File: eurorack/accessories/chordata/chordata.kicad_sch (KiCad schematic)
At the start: 44 parts, among them J1 USB_C_Receptacle_USB2.0, J2 Conn_02x05_Odd_Even, J3 Conn_01x18, J4 Conn_01x18, SW1 SW_Push, SW2 SW_Push, U1 MIC5219-3.3YM5, U2 RP2040, U3 W25Q128JVS, Y1 Crystal_GND24

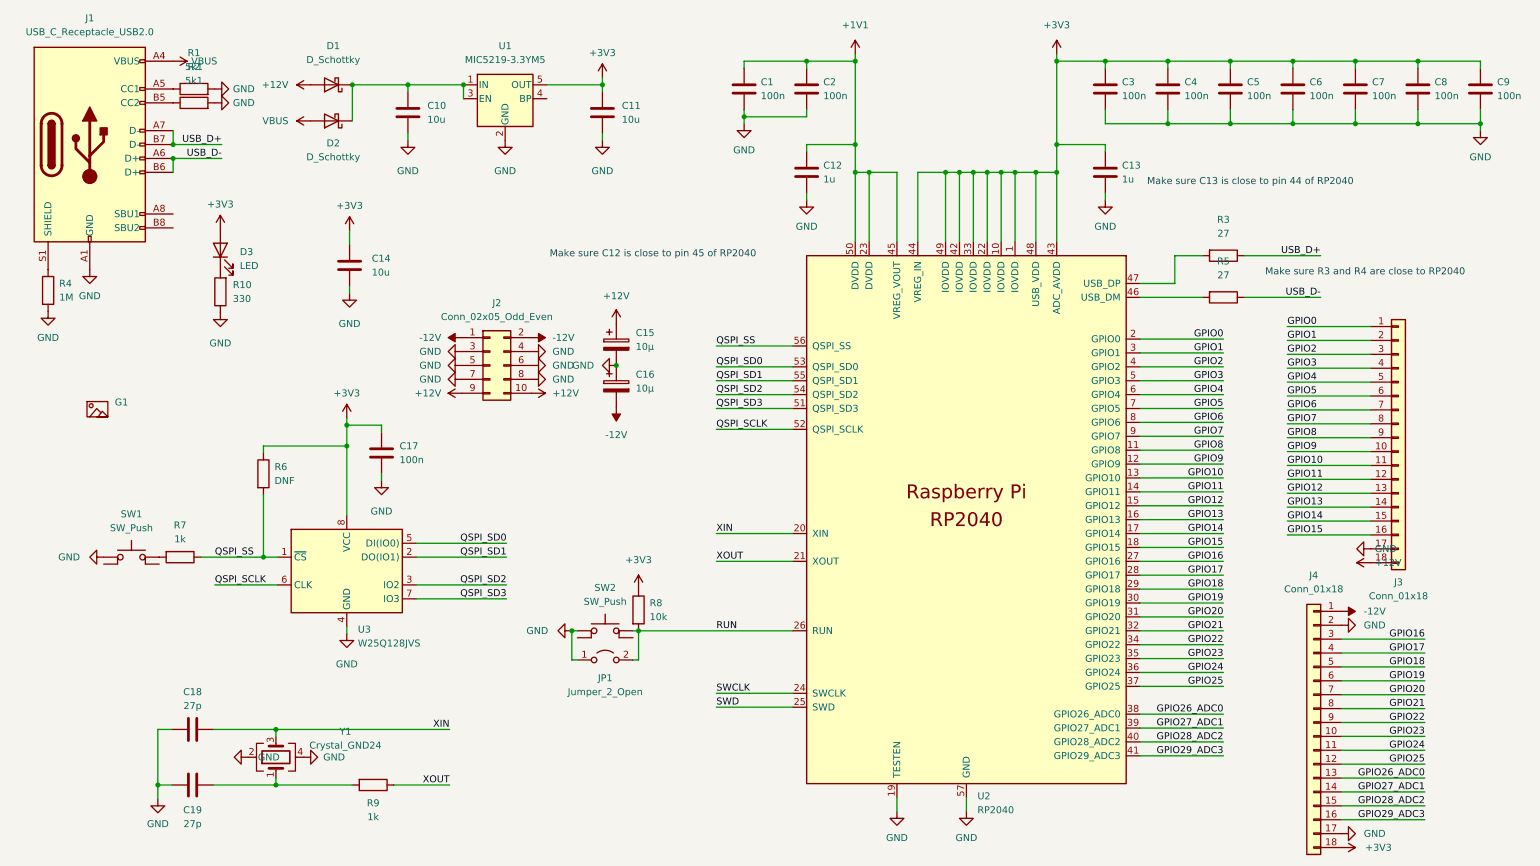
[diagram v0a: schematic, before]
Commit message: final chordata v1 layout
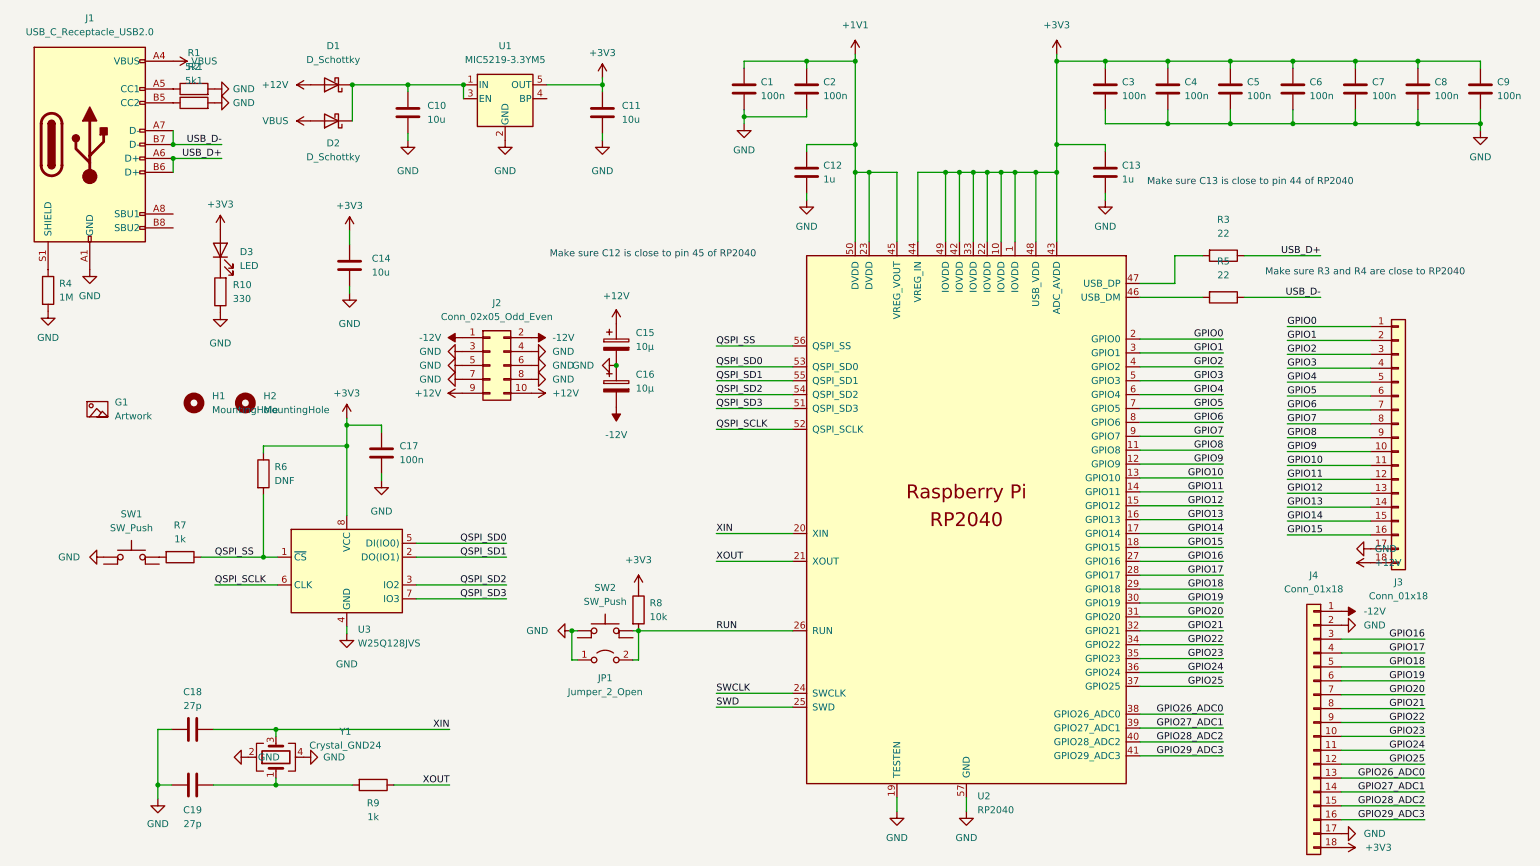
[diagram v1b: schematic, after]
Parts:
- added H1, H2: MountingHole, Pale Slim Ghost:hole JLCPCB tooling, symbol Mechanical:MountingHole
- C15, C16, J1, J2, J3, J4, JP1, R6, U1: now left out of the parts list
- D3: footprint LED_SMD:LED_0402_1005Metric -> LED_SMD:LED_0603_1608Metric
- G1: value (none) -> Artwork; footprint (none) -> Pale Slim Ghost:logo 12mm
- R3, R5: value 27 -> 22
- SW1, SW2: footprint Pale Slim Ghost:SW_Push_1P1T_NO_CK_KMR2 -> Pale Slim Ghost:SW_Push_1P1T_SKSGACE010; now left out of the parts list
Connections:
- net USB_D+: now also J1.A6 (D+), J1.B6 (D+); no longer J1.A7 (D-), J1.B7 (D-)
- net USB_D-: now also J1.A7 (D-), J1.B7 (D-); no longer J1.A6 (D+), J1.B6 (D+)

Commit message: chordata v2 final layout
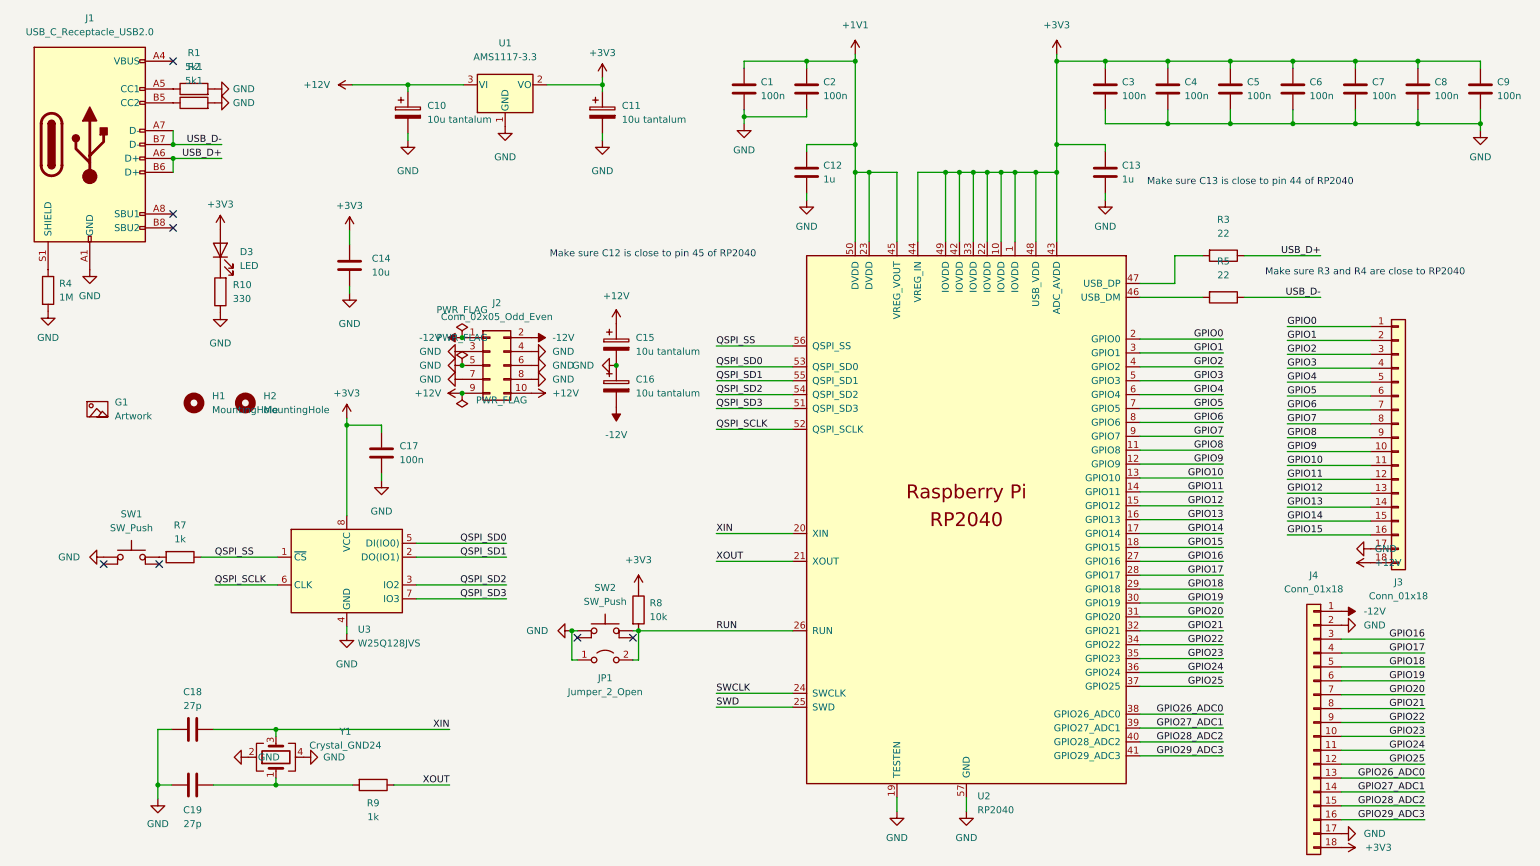
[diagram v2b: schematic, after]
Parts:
- removed C10: 10u, Capacitor_SMD:C_0805_2012Metric, symbol Device:C
- removed D1, D2: D_Schottky, Diode_SMD:D_SOD-123, symbol Device:D_Schottky
- removed R6: DNF, Resistor_SMD:R_0402_1005Metric, symbol Device:R
- removed U1: MIC5219-3.3YM5, Package_TO_SOT_SMD:SOT-23-5, symbol Regulator_Linear:MIC5219-3.3YM5
- added C10: 10u tantalum, Capacitor_Tantalum_SMD:CP_EIA-3216-18_Kemet-A, symbol Device:C_Polarized
- added U1: AMS1117-3.3, Package_TO_SOT_SMD:SOT-223-3_TabPin2, symbol Regulator_Linear:AMS1117-3.3
- C11: value 10u -> 10u tantalum; footprint Capacitor_SMD:C_0805_2012Metric -> Capacitor_Tantalum_SMD:CP_EIA-3216-18_Kemet-A; symbol Device:C -> Device:C_Polarized
- C15, C16: value 10μ -> 10u tantalum; footprint Capacitor_SMD:CP_Elec_5x4.5 -> Capacitor_Tantalum_SMD:CP_EIA-3216-18_Kemet-A; now in the parts list
- J1: footprint Connector_USB:USB_C_Receptacle_XKB_U262-16XN-4BVC11 -> Connector_USB:USB_C_Receptacle_GCT_USB4085
- SW1, SW2: footprint Pale Slim Ghost:SW_Push_1P1T_SKSGACE010 -> Pale Slim Ghost:SW_Push_1P1T_NO_CK_KMR2
- U2: footprint Package_DFN_QFN:QFN-56-1EP_7x7mm_P0.4mm_EP5.6x5.6mm_ThermalVias -> Package_DFN_QFN:QFN-56-1EP_7x7mm_P0.4mm_EP3.2x3.2mm_ThermalVias
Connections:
- net +12V: now also C10.1, U1.3 (VI)
- net +3V3: now also U1.2 (VO)
- net GND: now also C10.2, U1.1 (GND)
- net VBUS: no longer names the net of J1.A4 (VBUS), J1.A9 (VBUS), J1.B4 (VBUS), J1.B9 (VBUS)
- no-connect marks 0 -> 7
